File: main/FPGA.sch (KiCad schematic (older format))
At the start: 50 parts, among them IC3 ESP-PSRAM64H, J4 FPGA_debug, J5 FPGA_GPIO, U2 S25FL127S, U3 XC7A100T-FTG256, X1 FGPA_Oscillator

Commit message: Start PCB layout
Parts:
- C20: footprint (none) -> Capacitor_Tantalum_SMD:CP_EIA-7343-43_Kemet-X_Pad2.25x2.55mm_HandSolder
- IC3: Manufacturer_Name Espressif Systems -> Adafruit Industries; Manufacturer_Part_Number ESP-PSRAM64H -> 4677; URL (none) -> https://www.digikey.com/en/products/detail/adafruit-industr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
- J5: Manufacturer_Name (none) -> Multicomp PRO; Manufacturer_Part_Number (none) -> 2213S-50G; URL (none) -> https://no.farnell.com/multicomp/2213s-50g/connector-header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
- U2: Description (none) -> Flash for the FPGA; Manufacturer_Name (none) -> Cypress; Manufacturer_Part_Number (none) -> S25FL127SABMFV101; URL (none) -> https://no.farnell.com/cypress-semiconductor/s25fl127sabmfv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
- U3: Manufacturer_Name (none) -> Xilinx; Manufacturer_Part_Number (none) -> XC7A100T-FTG256
- X1: footprint (none) -> Oscillator:Oscillator_SMD_SeikoEpson_SG210-4Pin_2.5x2.0mm_HandSoldering
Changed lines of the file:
@@
 F 1 "XC7A100T-FTG256" H 1950 10976 50  0000 C CNN
 F 2 "Package_BGA:Xilinx_FTG256" H 1950 9500 50  0001 C CNN
-F 3 "" H 1950 9500 50  0000 C CNN
+F 3 "https://www.google.com/url?sa=t&rct=j&q=&esrc=s&source=web&cd=&cad=rja&uact=8&ved=2ahUKEwiH1rrnlZ_zAhUrtYsKHcsIDFQQFnoECAUQAQ&url=https%3A%2F%2Fwww.xilinx.com%2Fsupport%2Fdocumentation%2Fuser_guides%2Fug475_7Series_Pkg_Pinout.pdf&usg=AOvVaw3NyLHDtSbZv1hXp1wxMn0l" H 1950 9500 50  0000 C CNN
+F 4 "Xilinx" H 1950 9500 50  0001 C CNN "Manufacturer_Name"
+F 5 "XC7A100T-FTG256" H 1950 9500 50  0001 C CNN "Manufacturer_Part_Number"
 	4    1950 9500
 	1    0    0    -1
@@
 F 1 "XC7A100T-FTG256" H 6900 6850 50  0000 R CNN
 F 2 "Package_BGA:Xilinx_FTG256" H 7450 5400 50  0001 C CNN
-F 3 "" H 7450 5400 50  0000 C CNN
+F 3 "https://www.google.com/url?sa=t&rct=j&q=&esrc=s&source=web&cd=&cad=rja&uact=8&ved=2ahUKEwiH1rrnlZ_zAhUrtYsKHcsIDFQQFnoECAUQAQ&url=https%3A%2F%2Fwww.xilinx.com%2Fsupport%2Fdocumentation%2Fuser_guides%2Fug475_7Series_Pkg_Pinout.pdf&usg=AOvVaw3NyLHDtSbZv1hXp1wxMn0l" H 7450 5400 50  0000 C CNN
+F 4 "Xilinx" H 7450 5400 50  0001 C CNN "Manufacturer_Name"
+F 5 "XC7A100T-FTG256" H 7450 5400 50  0001 C CNN "Manufacturer_Part_Number"
 	3    7450 5400
 	-1   0    0    1
@@
 F 0 "C20" H 1400 7600 50  0000 L CNN
 F 1 "330uF" H 1400 7400 50  0000 L CNN
-F 2 "" H 1350 7500 50  0001 C CNN
+F 2 "Capacitor_Tantalum_SMD:CP_EIA-7343-43_Kemet-X_Pad2.25x2.55mm_HandSolder" H 1350 7500 50  0001 C CNN
 F 3 "~" H 1350 7500 50  0001 C CNN
 	1    1350 7500
@@
 F 2 "Package_SO:SOIC-8_5.275x5.275mm_P1.27mm" H 4250 3250 50  0001 C CNN
 F 3 "https://www.farnell.com/datasheets/2330438.pdf" H 4250 3250 50  0001 C CNN
+F 4 "Flash for the FPGA" H 4700 3200 50  0001 C CNN "Description"
+F 5 "Cypress" H 4700 3200 50  0001 C CNN "Manufacturer_Name"
+F 6 "S25FL127SABMFV101" H 4700 3200 50  0001 C CNN "Manufacturer_Part_Number"
+F 7 "https://no.farnell.com/cypress-semiconductor/s25fl127sabmfv101/flash-memory-128mbit-108mhz-soic/dp/2772749?st=s25fl127s" H 4700 3200 50  0001 C CNN "URL"
 	1    4700 3200
 	1    0    0    -1
@@
 F 1 "ESP-PSRAM64H" H 10450 9950 50  0000 C CNN
 F 2 "ESP-PSRAM64H:SOIC127P600X175-8N" H 11100 10500 50  0001 L CNN
-F 3 "https://www.espressif.com/sites/default/files/documentation/esp-psram64_esp-psram64h_datasheet_en.pdf" H 11100 10400 50  0001 L CNN
+F 3 "https://cdn-shop.adafruit.com/product-files/4677/4677_esp-psram64_esp-psram64h_datasheet_en.pdf" H 11100 10400 50  0001 L CNN
 F 4 "ESP-PSRAM64 and ESP-PSRAM64H 64 Mbit serial pseudo SRAM" H 11100 10300 50  0001 L CNN "Description"
 F 5 "1.75" H 11100 10200 50  0001 L CNN "Height"
-F 6 "Espressif Systems" H 11100 10100 50  0001 L CNN "Manufacturer_Name"
-F 7 "ESP-PSRAM64H" H 11100 10000 50  0001 L CNN "Manufacturer_Part_Number"
+F 6 "Adafruit Industries" H 11100 10100 50  0001 L CNN "Manufacturer_Name"
+F 7 "4677" H 11100 10000 50  0001 L CNN "Manufacturer_Part_Number"
 F 8 "" H 11100 9900 50  0001 L CNN "Mouser Part Number"
 F 9 "" H 11100 9800 50  0001 L CNN "Mouser Price/Stock"
 F 10 "" H 11100 9700 50  0001 L CNN "Arrow Part Number"
 F 11 "" H 11100 9600 50  0001 L CNN "Arrow Price/Stock"
+F 12 "https://www.digikey.com/en/products/detail/adafruit-industries-llc/4677/13148775" H 9650 10400 50  0001 C CNN "URL"
 	1    9650 10400
 	1    0    0    -1
@@
 F 1 "XC7A100T-FTG256" H 13900 900 50  0000 C CNN
 F 2 "Package_BGA:Xilinx_FTG256" H 13900 3850 50  0001 C CNN
-F 3 "" H 13900 3850 50  0000 C CNN
+F 3 "https://www.google.com/url?sa=t&rct=j&q=&esrc=s&source=web&cd=&cad=rja&uact=8&ved=2ahUKEwiH1rrnlZ_zAhUrtYsKHcsIDFQQFnoECAUQAQ&url=https%3A%2F%2Fwww.xilinx.com%2Fsupport%2Fdocumentation%2Fuser_guides%2Fug475_7Series_Pkg_Pinout.pdf&usg=AOvVaw3NyLHDtSbZv1hXp1wxMn0l" H 13900 3850 50  0000 C CNN
+F 4 "Xilinx" H 13900 3850 50  0001 C CNN "Manufacturer_Name"
+F 5 "XC7A100T-FTG256" H 13900 3850 50  0001 C CNN "Manufacturer_Part_Number"
 	1    13900 3850
 	1    0    0    -1
@@
 F 1 "FPGA_GPIO" H 13450 8026 50  0000 C CNN
 F 2 "Connector_PinHeader_2.54mm:PinHeader_2x06_P2.54mm_Vertical" H 13400 7700 50  0001 C CNN
-F 3 "~" H 13400 7700 50  0001 C CNN
+F 3 "https://www.farnell.com/datasheets/3029611.pdf" H 13400 7700 50  0001 C CNN
+F 4 "Multicomp PRO" H 13400 7700 50  0001 C CNN "Manufacturer_Name"
+F 5 "2213S-50G" H 13400 7700 50  0001 C CNN "Manufacturer_Part_Number"
+F 6 "https://no.farnell.com/multicomp/2213s-50g/connector-header-50pos-2-54mm/dp/2847228" H 13400 7700 50  0001 C CNN "URL"
 	1    13400 7700
 	-1   0    0    -1
@@
 F 1 "XC7A100T-FTG256" H 18800 734 50  0000 C CNN
 F 2 "Package_BGA:Xilinx_FTG256" H 18800 3800 50  0001 C CNN
-F 3 "" H 18800 3800 50  0000 C CNN
+F 3 "https://www.google.com/url?sa=t&rct=j&q=&esrc=s&source=web&cd=&cad=rja&uact=8&ved=2ahUKEwiH1rrnlZ_zAhUrtYsKHcsIDFQQFnoECAUQAQ&url=https%3A%2F%2Fwww.xilinx.com%2Fsupport%2Fdocumentation%2Fuser_guides%2Fug475_7Series_Pkg_Pinout.pdf&usg=AOvVaw3NyLHDtSbZv1hXp1wxMn0l" H 18800 3800 50  0000 C CNN
+F 4 "Xilinx" H 18800 3800 50  0001 C CNN "Manufacturer_Name"
+F 5 "XC7A100T-FTG256" H 18800 3800 50  0001 C CNN "Manufacturer_Part_Number"
 	2    18800 3800
 	1    0    0    -1
@@
 F 0 "X1" H 8844 7996 50  0000 L CNN
 F 1 "FGPA_Oscillator" H 8844 7905 50  0000 L CNN
-F 2 "" H 9200 7600 50  0001 C CNN
+F 2 "Oscillator:Oscillator_SMD_SeikoEpson_SG210-4Pin_2.5x2.0mm_HandSoldering" H 9200 7600 50  0001 C CNN
 F 3 "http://www.txccorp.com/download/products/osc/7C_o.pdf" H 8400 7950 50  0001 C CNN
+F 4 "" H 8500 7950 50  0001 C CNN "URL"
 	1    8500 7950
 	1    0    0    -1

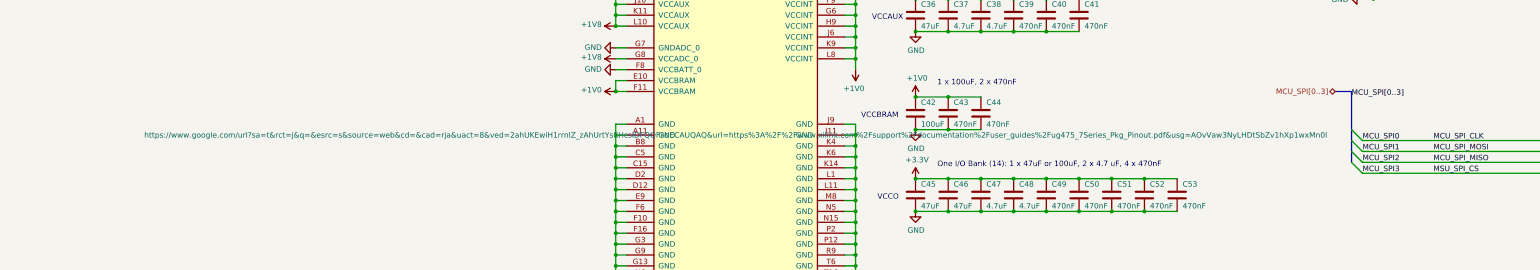
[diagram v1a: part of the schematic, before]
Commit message: Continue PCB layout
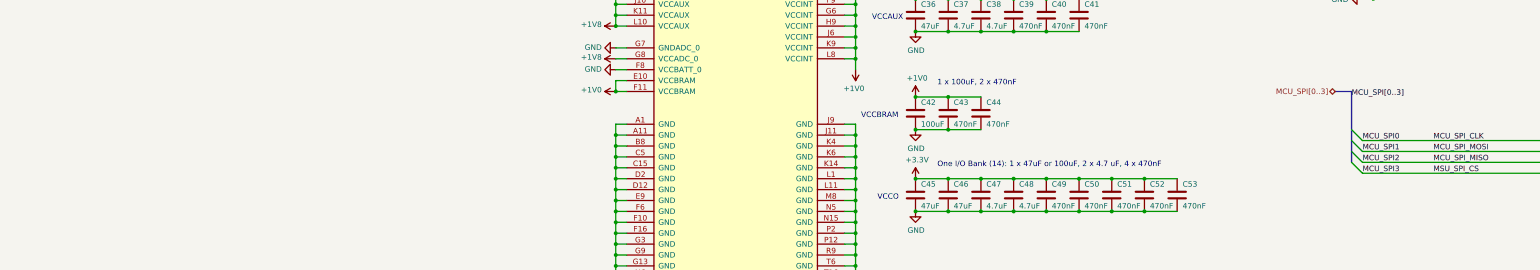
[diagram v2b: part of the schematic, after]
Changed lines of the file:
@@
 F 1 "XC7A100T-FTG256" H 1950 10976 50  0000 C CNN
 F 2 "Package_BGA:Xilinx_FTG256" H 1950 9500 50  0001 C CNN
-F 3 "https://www.google.com/url?sa=t&rct=j&q=&esrc=s&source=web&cd=&cad=rja&uact=8&ved=2ahUKEwiH1rrnlZ_zAhUrtYsKHcsIDFQQFnoECAUQAQ&url=https%3A%2F%2Fwww.xilinx.com%2Fsupport%2Fdocumentation%2Fuser_guides%2Fug475_7Series_Pkg_Pinout.pdf&usg=AOvVaw3NyLHDtSbZv1hXp1wxMn0l" H 1950 9500 50  0000 C CNN
+F 3 "https://www.google.com/url?sa=t&rct=j&q=&esrc=s&source=web&cd=&cad=rja&uact=8&ved=2ahUKEwiH1rrnlZ_zAhUrtYsKHcsIDFQQFnoECAUQAQ&url=https%3A%2F%2Fwww.xilinx.com%2Fsupport%2Fdocumentation%2Fuser_guides%2Fug475_7Series_Pkg_Pinout.pdf&usg=AOvVaw3NyLHDtSbZv1hXp1wxMn0l" H 1950 9500 50  0001 C CNN
 F 4 "Xilinx" H 1950 9500 50  0001 C CNN "Manufacturer_Name"
 F 5 "XC7A100T-FTG256" H 1950 9500 50  0001 C CNN "Manufacturer_Part_Number"
